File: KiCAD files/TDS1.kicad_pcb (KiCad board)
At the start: 2 copper layers, 40.6 x 50 mm, 16 parts, among them J1 Conn_01x02_Pin, J2 Conn_01x02_Pin, J3 Conn_01x02_Pin, U1 TL072

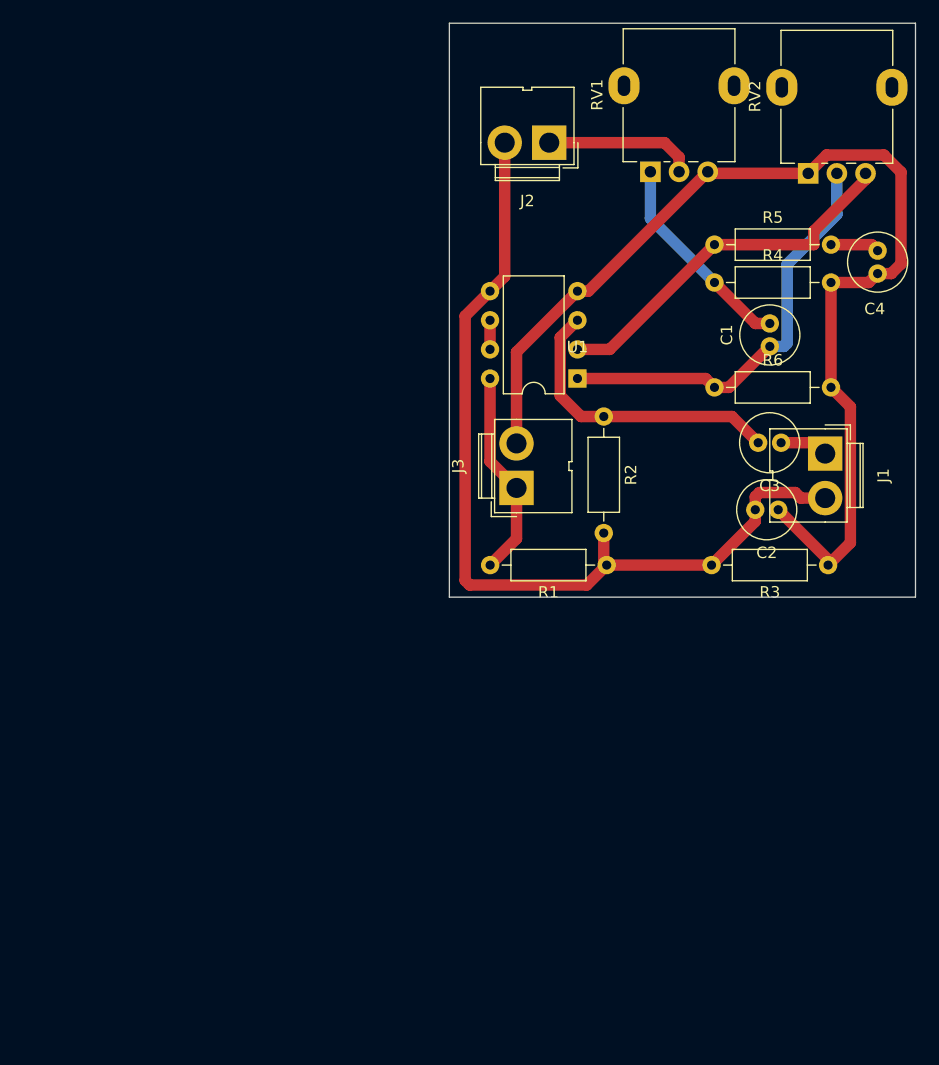
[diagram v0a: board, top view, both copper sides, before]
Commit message: pcb and schematic
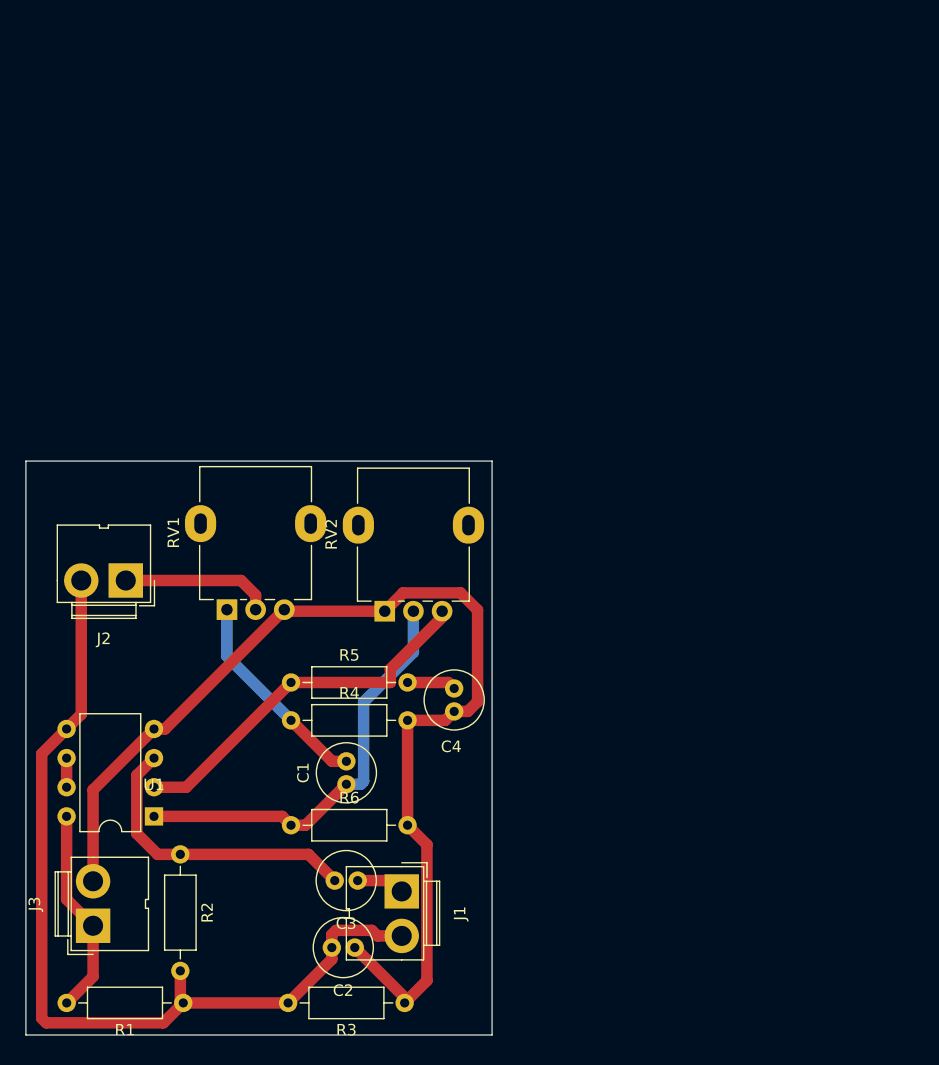
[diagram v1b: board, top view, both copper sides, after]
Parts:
- moved C1 53.1 mm to (157.6, 99.4)
- moved C2 53.1 mm to (158.4, 113.6)
- moved C3 53.1 mm to (158.6, 107.8)
- moved J2 53.1 mm to (138.4, 81.6)
- moved J3 53.1 mm to (135.6, 111.7)
- moved R1 53.1 mm to (143.4, 118.4)
- moved R2 53.1 mm to (143.2, 105.5)
- moved R3 53.1 mm to (162.7, 118.4)
- moved R4 53.1 mm to (152.8, 93.8)
- moved R5 53.1 mm to (152.8, 90.5)
- moved R6 53.1 mm to (152.8, 102.9)
- moved RV1 53.1 mm to (147.2, 84.1)
- moved C4 53.1 mm to (167.0, 93.0)
- moved J1 53.1 mm to (162.5, 108.7)
- moved RV2 53.1 mm to (161.0, 84.3)
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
